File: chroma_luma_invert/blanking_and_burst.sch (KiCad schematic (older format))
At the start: 28 parts, among them U10 74HC4538, U5 LM311, U6 LM311, U7 74HC4538, U8 74HC4538, U9 4040

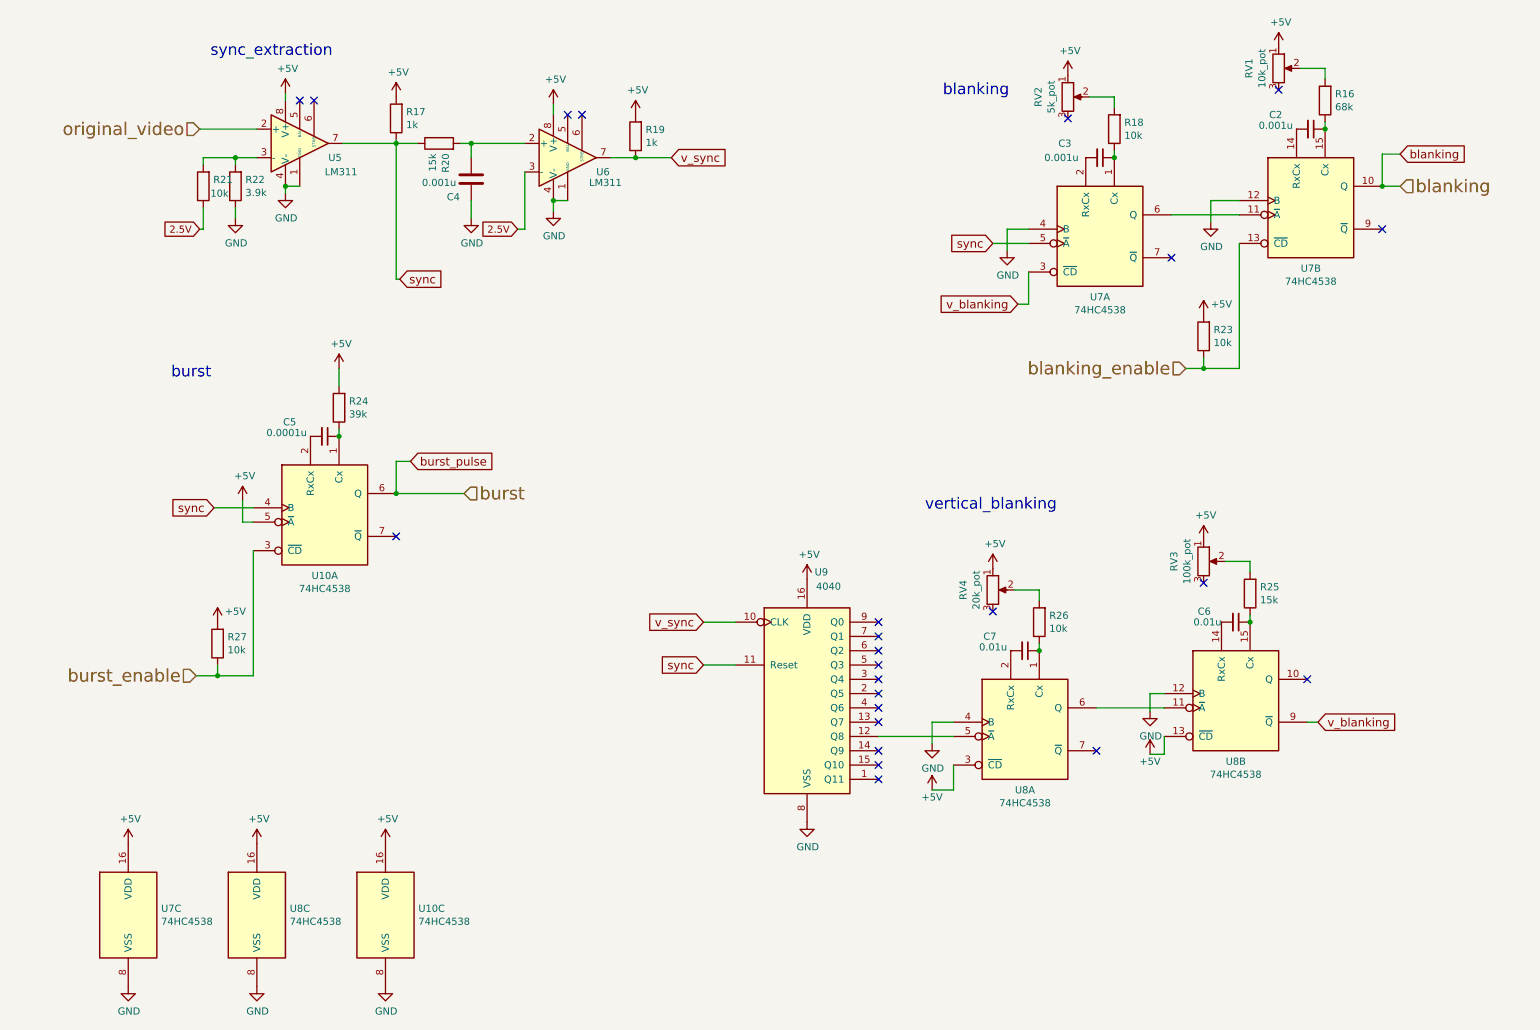
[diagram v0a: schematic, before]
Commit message: updated two_comparator and added two_point_one
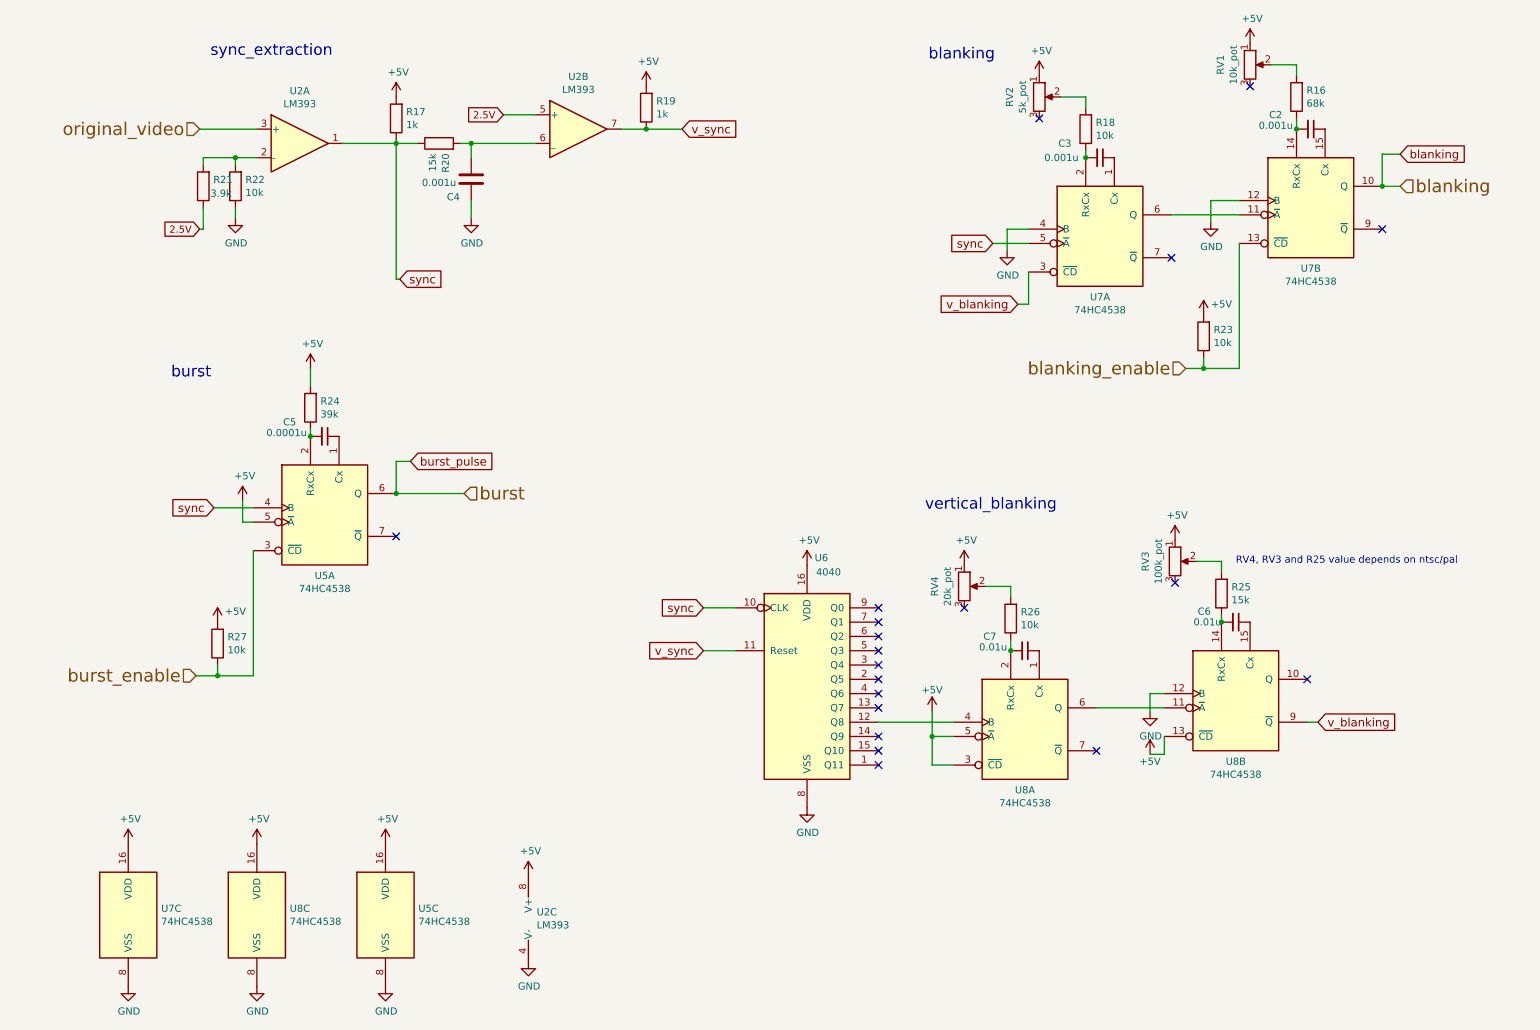
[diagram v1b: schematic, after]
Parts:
- removed U5, U6: LM311, Package_DIP:DIP-8_W7.62mm_LongPads, symbol Comparator:LM311
- added U2: LM393, Package_DIP:DIP-8_W7.62mm_LongPads, symbol Comparator:LM393
- R21: value 10k -> 3.9k
- R22: value 3.9k -> 10k
- renumbered U10 to U5, U9 to U6
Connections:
- net +5V: now also U8.5 (~A), U2.8 (V+)
- net 2.5V: now also U2.5 (+)
- net GND: now also U2.4 (V-); no longer U8.4 (B)
- net original_video: now also U2.3 (+)
- net sync: now also U6.10 (CLK), U2.1; no longer U6.11 (Reset)
- net v_sync: now also U6.11 (Reset), U2.7; no longer U6.10 (CLK)
- net at R21.2, R22.2: now also U2.2 (-)
- net at C3.1, U7.1 (Cx): no longer R18.1
- net at C3.2, U7.2 (RxCx): now also R18.1
- net at C4.2, R20.2: now also U2.6 (_)
- net at C2.1, U7.15 (Cx): no longer R16.1
- net at C2.2, U7.14 (RxCx): now also R16.1
- net at U6.12 (Q8): now also U8.4 (B); no longer U8.5 (~A)
- net at C7.1, U8.1 (Cx): no longer R26.1
- net at C7.2, U8.2 (RxCx): now also R26.1
- net at C6.1, U8.15 (Cx): no longer R25.1
- net at C6.2, U8.14 (RxCx): now also R25.1
- net at C5.1, U5.1 (Cx): no longer R24.1
- net at C5.2, U5.2 (RxCx): now also R24.1
- no-connect marks 24 -> 20
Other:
- note added: "RV4, RV3 and R25 value depends on ntsc/pal"
- moved on the sheet: R16, R18, R19, R24, R25, R26, RV1, RV2, RV3, RV4, U6
